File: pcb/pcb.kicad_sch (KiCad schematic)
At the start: 51 parts, among them J1 N!N, J2 Conn_01x02_Socket, J3 Conn_01x12_Socket, J4 Display_nice-view, J5 Conn_01x12_Socket, J6 Conn_01x12_Socket, J7 Conn_01x12_Socket, SW10 Switch, SW11 Switch, SW12 Switch, SW13 Switch, SW14 Switch, SW15 Switch, SW18 Switch, SW19 Switch, SW21 SW_Push, SW22 SW_SPDT, SW3 Switch, SW4 Switch, SW5 Switch, SW6 Switch, SW7 Switch, SW8 Switch, SW9 Switch

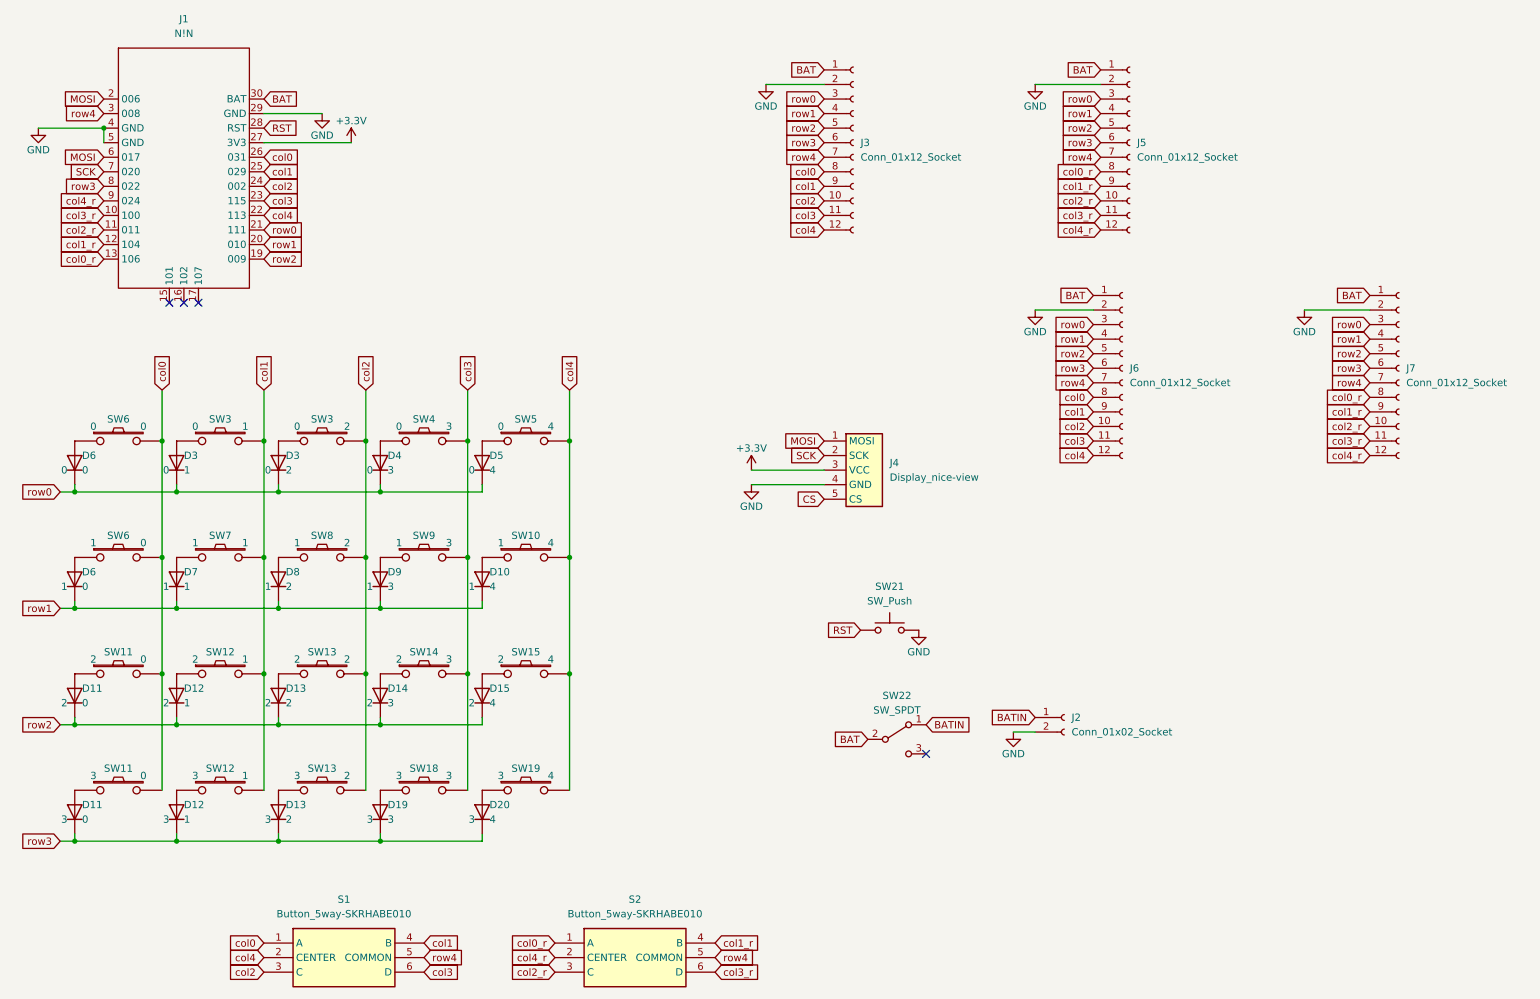
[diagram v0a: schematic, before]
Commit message: final pcb
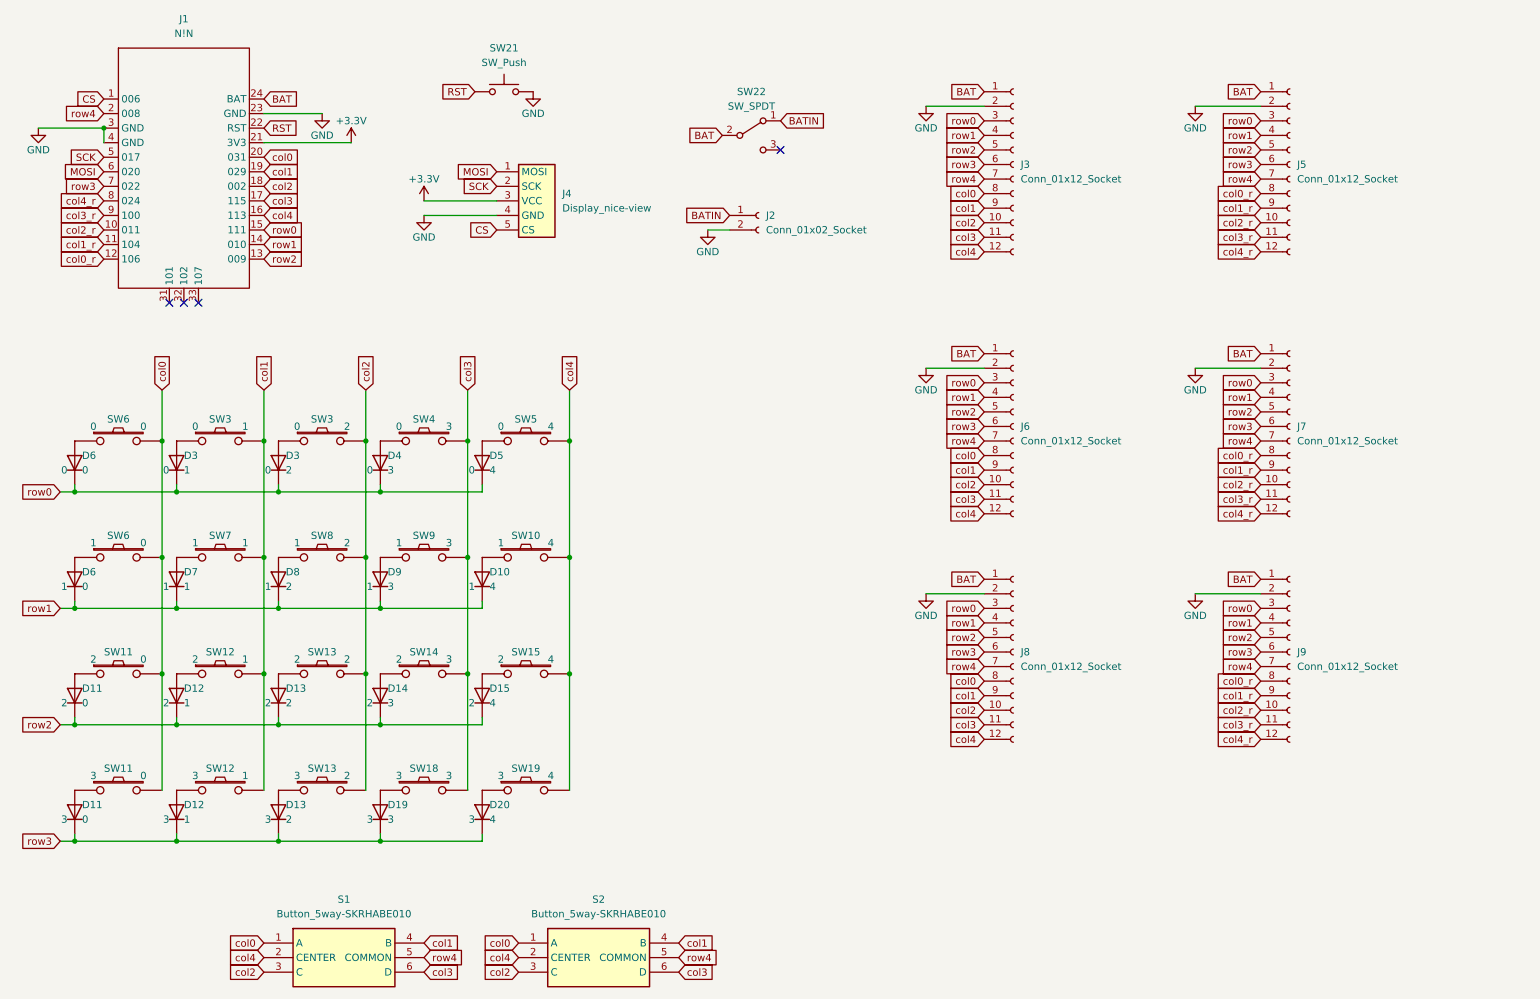
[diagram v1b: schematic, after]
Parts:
- added J8, J9: Conn_01x12_Socket, Connector_FFC-FPC:TE_1-84952-2_1x12-1MP_P1.0mm_Horizontal, symbol Connector:Conn_01x12_Socket
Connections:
- net +3.3V: now also J1.21 (3V3); no longer J1.27 (3V3)
- net BAT: now also J1.24 (BAT), J8.1 (Pin_1), J9.1 (Pin_1); no longer J1.30 (BAT)
- net CS: now also J1.1 (006)
- net GND: now also J1.23 (GND), J1.3 (GND), J8.2 (Pin_2), J9.2 (Pin_2); no longer J1.29 (GND), J1.5 (GND)
- net MOSI: no longer J1.2 (006)
- net RST: now also J1.22 (RST); no longer J1.28 (RST)
- net SCK: now also J1.5 (017); no longer J1.7 (020)
- net col0: now also J1.20 (031), S2.1 (A), J8.8 (Pin_8); no longer J1.26 (031)
- net col0_r: now also J1.12 (106), J9.8 (Pin_8); no longer J1.13 (106), S2.1 (A)
- net col1: now also J1.19 (029), S2.4 (B), J8.9 (Pin_9); no longer J1.25 (029)
- net col1_r: now also J1.11 (104), J9.9 (Pin_9); no longer J1.12 (104), S2.4 (B)
- net col2: now also J1.18 (002), S2.3 (C), J8.10 (Pin_10); no longer J1.24 (002)
- net col2_r: now also J1.10 (011), J9.10 (Pin_10); no longer J1.11 (011), S2.3 (C)
- net col3: now also J1.17 (115), S2.6 (D), J8.11 (Pin_11); no longer J1.23 (115)
- net col3_r: now also J1.9 (100), J9.11 (Pin_11); no longer J1.10 (100), S2.6 (D)
- net col4: now also J1.16 (113), S2.2 (CENTER), J8.12 (Pin_12); no longer J1.22 (113)
- net col4_r: now also J1.8 (024), J9.12 (Pin_12); no longer J1.9 (024), S2.2 (CENTER)
- net row0: now also J1.15 (111), J8.3 (Pin_3), J9.3 (Pin_3); no longer J1.21 (111)
- net row1: now also J1.14 (010), J8.4 (Pin_4), J9.4 (Pin_4); no longer J1.20 (010)
- net row2: now also J1.13 (009), J8.5 (Pin_5), J9.5 (Pin_5); no longer J1.19 (009)
- net row3: now also J1.7 (022), J8.6 (Pin_6), J9.6 (Pin_6); no longer J1.8 (022)
- net row4: now also J1.2 (008), J8.7 (Pin_7), J9.7 (Pin_7); no longer J1.3 (008)
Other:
- moved on the sheet: J2, J3, J4, J5, J6, J7, SW21, SW22
